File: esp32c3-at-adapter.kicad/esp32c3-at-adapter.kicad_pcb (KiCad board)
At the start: 2 copper layers, 6 parts, among them J1 Grove, J2 Conn_01x02, U1 ESP32-C3_SUPERMINI

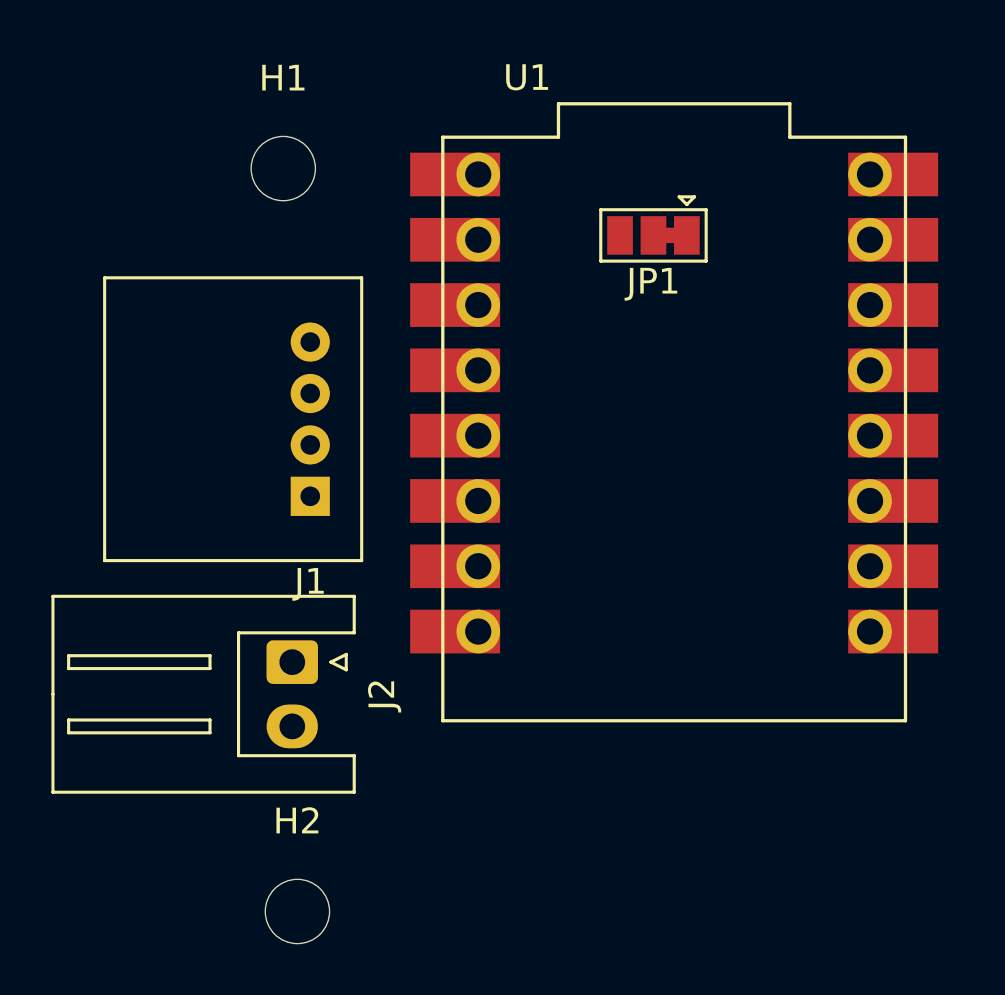
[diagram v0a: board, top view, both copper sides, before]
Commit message: Rev: 0.90 (first production test)
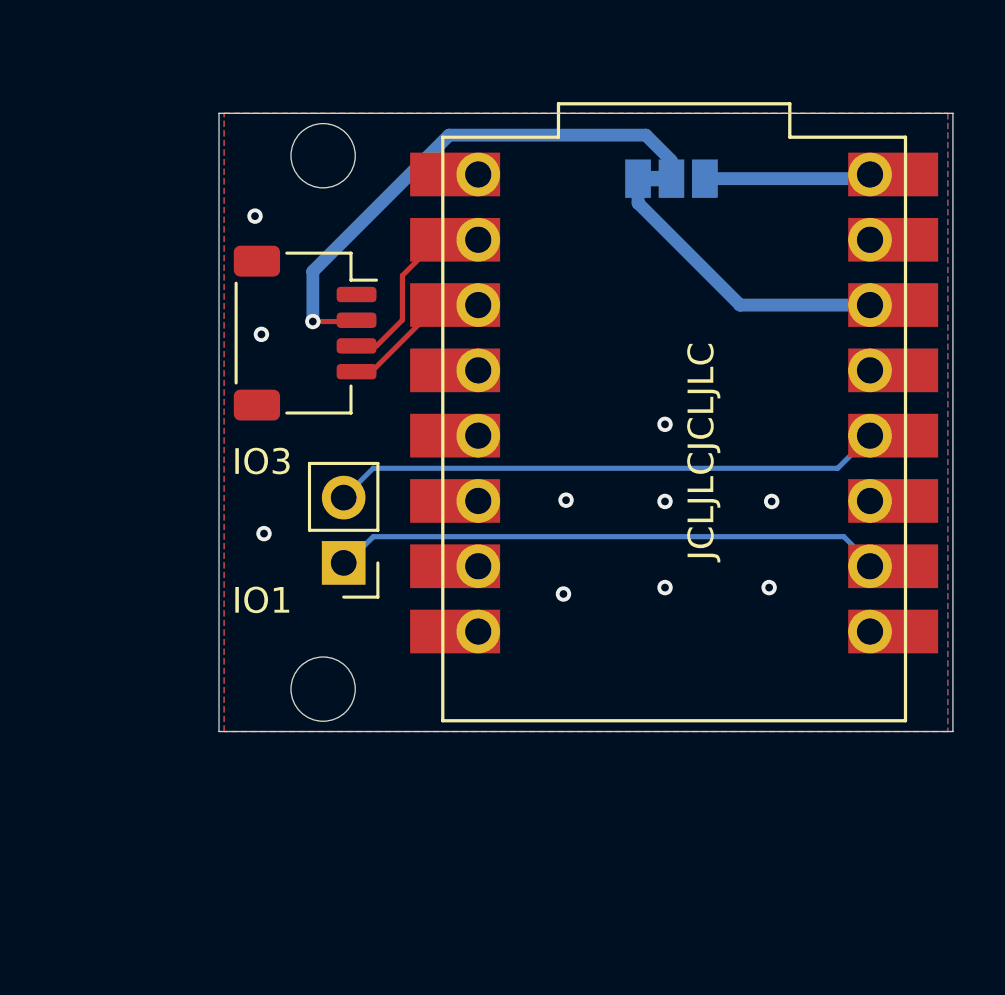
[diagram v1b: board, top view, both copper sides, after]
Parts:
- J1: value Grove -> Stemma-QT_Qwicc; footprint user:Grove_1x04_P2mm_Horizontal -> user:JST_SH_SM04B-SRSS-TB_1x04-1MP_P1.00mm_Horizontal
- J2: value Conn_01x02 -> WakePins; footprint Connector_JST:JST_XH_S2B-XH-A_1x02_P2.50mm_Horizontal -> Connector_PinHeader_2.54mm:PinHeader_1x02_P2.54mm_Vertical
- JP1: value Jumper_3_Bridged12 -> PWR_Select; moved to B.Cu
- moved H2 8.71 mm to (135.7, 93.0)
- moved J2 4.35 mm to (136.5, 88.1), turned to 180 degrees
- moved J1 3.36 mm to (135.0, 79.2), turned to -90 degrees
- moved JP1 2.32 mm to (149.2, 73.1), turned to 0 degrees
- moved H1 1.63 mm to (135.7, 72.2)
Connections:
- J1 pad 1: /ESP_TX -> GND
- J1 pad 2: /ESP_RX -> VCC
- J1 pad 3: VCC -> /ESP_RX
- J1 pad 4: GND -> /ESP_TX
- JP1 pad 1: VCC -> +3V3
- JP1 pad 2: +3V3 -> VCC
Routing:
- net /GPIO3: track 0.00 -> 21.5 mm
- net /GPIO1: track 0.00 -> 21.4 mm
- net VCC: track 0.00 -> 20.2 mm, vias 0 -> 1
- net +3V3: track 0.00 -> 11.6 mm
- net /ESP_RX: track 0.00 -> 7.46 mm
- net +5V: track 0.00 -> 6.49 mm
- net /ESP_TX: track 0.00 -> 5.81 mm
- net GND: vias 0 -> 10
- added copper zone on B.Cu, net GND
- added copper zone on F.Cu, net GND
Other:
- board outline added: 28.5 x 24.1 mm
- board text added: "3V3"
- board text added: "5V"
- board text added: "GND"
- board text added: "IO0"
- board text added: "IO1"
- board text added: "IO10"
- board text added: "IO2"
- board text added: "IO20"
- board text added: "IO21"
- board text added: "IO3"
- board text added: "IO4"
- board text added: "IO5"
- board text added: "IO6"
- board text added: "IO7"
- board text added: "IO8"
- board text added: "IO9"
- board text added: "JCLJLCJCLJLC"
- board text added: "Rev: 0.90"
- board text added: "https://github.com/ bablokb/ esp32c3-at-adapter"
